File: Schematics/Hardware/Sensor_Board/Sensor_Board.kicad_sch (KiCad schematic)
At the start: 88 parts, among them U5 LCD

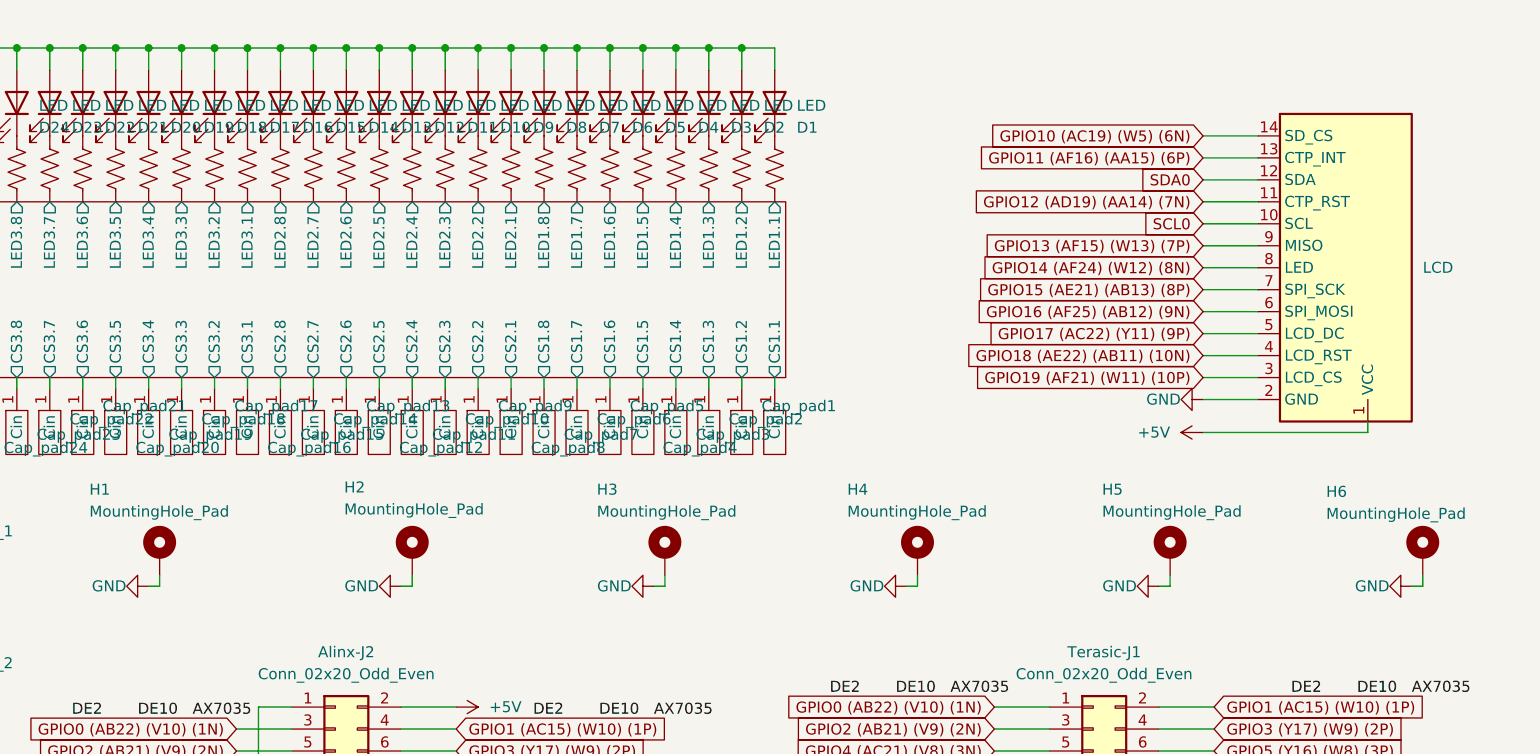
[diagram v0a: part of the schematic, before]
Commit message: Added
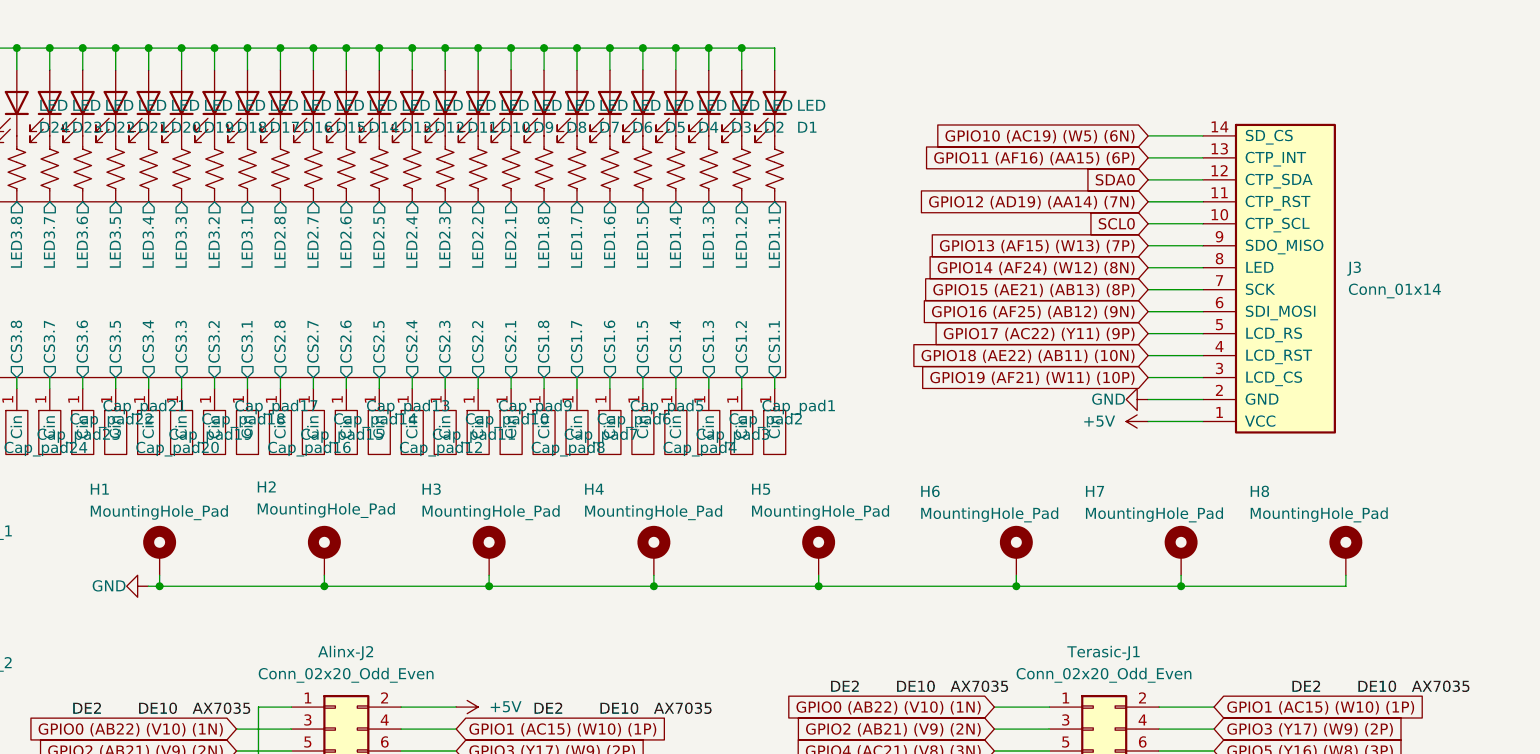
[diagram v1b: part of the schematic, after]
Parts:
- removed U5: LCD, Connector_PinSocket_2.54mm:PinSocket_1x14_P2.54mm_Vertical, symbol Symbols:LCD240X320
- added H7, H8: MountingHole_Pad, MountingHole:MountingHole_2.5mm_Pad_Via, symbol Mechanical:MountingHole_Pad
- added J3: Conn_01x14, Connector_PinSocket_2.54mm:PinSocket_1x14_P2.54mm_Vertical, symbol Connector_Generic:Conn_01x14
- Qwiic_1, Qwiic_2: footprint Connector_JST:JST_SH_BM04B-SRSS-TB_1x04-1MP_P1.00mm_Vertical -> Connector_JST:JST_SH_SM04B-SRSS-TB_1x04-1MP_P1.00mm_Horizontal
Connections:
- net +5V: now also J3.1 (VCC)
- net GND: now also H7.1, H8.1, J3.2 (GND)
- net GPIO10 (AC19) (W5) (6N): now also J3.14 (SD_CS)
- net GPIO11 (AF16) (AA15) (6P): now also J3.13 (CTP_INT)
- net GPIO12 (AD19) (AA14) (7N): now also J3.11 (CTP_RST)
- net GPIO13 (AF15) (W13) (7P): now also J3.9 (SDO_MISO)
- net GPIO14 (AF24) (W12) (8N): now also J3.8 (LED)
- net GPIO15 (AE21) (AB13) (8P): now also J3.7 (SCK)
- net GPIO16 (AF25) (AB12) (9N): now also J3.6 (SDI_MOSI)
- net GPIO17 (AC22) (Y11) (9P): now also J3.5 (LCD_RS)
- net GPIO18 (AE22) (AB11) (10N): now also J3.4 (LCD_RST)
- net GPIO19 (AF21) (W11) (10P): now also J3.3 (LCD_CS)
- net GPIO2 (AB21) (V9) (2N): now also J3.10 (CTP_SCL)
- net GPIO3 (Y17) (W9) (2P): now also J3.12 (CTP_SDA)
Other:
- moved on the sheet: H2, H3, H4, H5, H6
